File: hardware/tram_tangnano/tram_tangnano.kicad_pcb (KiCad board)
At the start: 4 copper layers, 93 x 26.7 mm, 61 parts, among them J1 Conn_01x01_SolderingPad, J10 Conn_01x01_SolderingPad, J11 Conn_01x01_SolderingPad, J12 Conn_01x01_SolderingPad, J13 Conn_01x01_SolderingPad, J14 Conn_01x01_SolderingPad, J15 Conn_01x01_SolderingPad, J16 Conn_01x01_SolderingPad, J17 Conn_01x01_SolderingPad, J18 Conn_01x01_SolderingPad, J19 Conn_01x01_SolderingPad, J2 Conn_01x01_SolderingPad, J20 Conn_01x01_SolderingPad, J21 Conn_01x01_SolderingPad, J22 Conn_01x01_SolderingPad, J23 Conn_01x01_SolderingPad, J24 Conn_01x01_SolderingPad, J3 Conn_01x04_Voltage, J4 Conn_01x01_SolderingPad, J5 Conn_01x01_SolderingPad, J6 Conn_01x01_SolderingPad, J7 Conn_01x01_SolderingPad, J8 Conn_01x01_SolderingPad, J9 Conn_01x01_SolderingPad, U1 Tang_Nano_20K, U10 TXU0202, U11 TXU0202, U12 TXU0202, U13 TXU0202, U20 TRAM, U4 SN74LVC2GU04, U6 SN74LVC1G06, U7 SN74LVC1G04

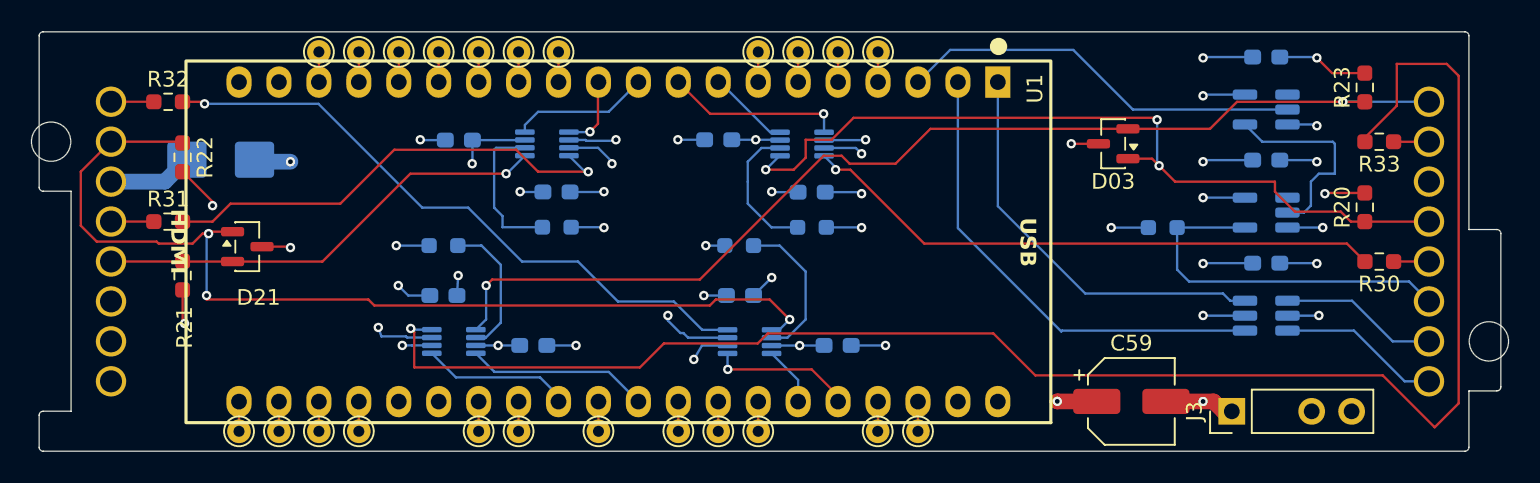
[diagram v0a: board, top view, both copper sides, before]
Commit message: temp
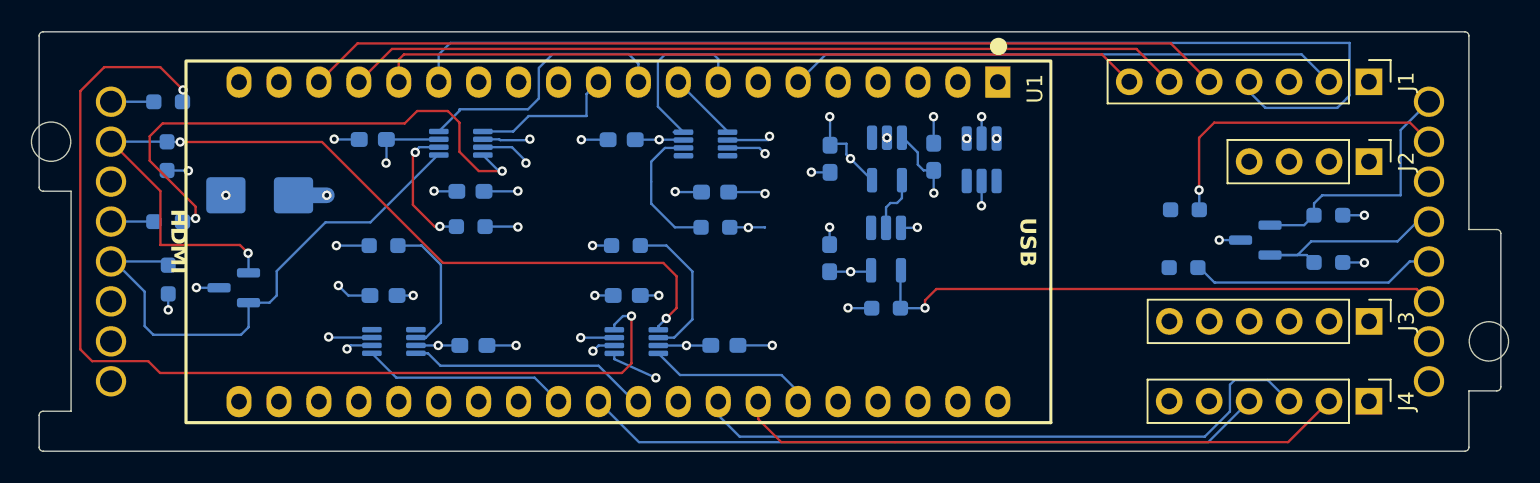
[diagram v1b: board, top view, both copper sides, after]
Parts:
- removed C59: 100µF, Capacitor_SMD:CP_Elec_5x3.9
- removed J10, J11, J12, J13, J14, J15, J16, J17, J18, J19, J20, J21, J22, J23, J24, J5, J6, J7, J8, J9: Conn_01x01_SolderingPad, Transputer:TestPoint_THTPad_D1.5mm_Drill0.7mm
- D03, D21, R20, R21, R22, R23, R30, R31, R32, R33: moved to B.Cu
- J1: value Conn_01x01_SolderingPad -> Conn_LED; footprint Transputer:TestPoint_THTPad_D1.5mm_Drill0.7mm -> Connector_PinHeader_2.54mm:PinHeader_1x07_P2.54mm_Vertical
- J2: value Conn_01x01_SolderingPad -> Conn_Event; footprint Transputer:TestPoint_THTPad_D1.5mm_Drill0.7mm -> Connector_PinHeader_2.54mm:PinHeader_1x04_P2.54mm_Vertical
- J3: value Conn_01x04_Voltage -> Conn_Link; footprint Transputer:PinHeader_1x04_P2.54mm_without_2 -> Connector_PinHeader_2.54mm:PinHeader_1x06_P2.54mm_Vertical
- J4: value Conn_01x01_SolderingPad -> Conn_Audio; footprint Transputer:TestPoint_THTPad_D1.5mm_Drill0.7mm -> Connector_PinHeader_2.54mm:PinHeader_1x06_P2.54mm_Vertical
- moved J4 38.9 mm to (214.6, 103.5), turned to -90 degrees
- moved J1 36.3 mm to (214.6, 83.2), turned to -90 degrees
- moved J2 35.6 mm to (214.6, 88.2), turned to -90 degrees
- moved C35 28.5 mm to (180.3, 88.1), turned to -90 degrees
- moved C34 28.5 mm to (180.3, 94.4), turned to 90 degrees
- moved U7 24.3 mm to (183.9, 88.1), turned to -90 degrees
- moved U6 24.3 mm to (183.9, 93.8), turned to -90 degrees
- moved C36 22.1 mm to (186.9, 87.9), turned to -90 degrees
- moved U4 20.6 mm to (190.0, 88.1), turned to 90 degrees
- moved R1 18.3 mm to (183.9, 97.6)
- moved R33 13.1 mm to (202.9, 91.3)
- moved R30 12.5 mm to (202.8, 95.0)
- moved D03 10.9 mm to (207.4, 93.2)
- moved J3 10.4 mm to (214.6, 98.4), turned to -90 degrees
- moved R23 8.45 mm to (212.0, 91.7), turned to 0 degrees
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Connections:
- net Net-(U1-25_IOB6A) renamed /ExtLink1In
- net Net-(U1-26_IOB6B) renamed /ExtLink1Out
- net Net-(U1-27_IOB8A) renamed /ExtLink0In
- net Net-(U1-28_IOB8B) renamed /ExtLink0Out
- net Net-(U1-41_IOB43A) renamed /ExtLink3In
- net Net-(U1-42_IOB42B) renamed /ExtLink3Out
- net Net-(U1-48_IOR49B) renamed /ExtLink4In
- net Net-(U1-49_IOR49A) renamed /ExtLink4Out
- J1 pad 1: Net-(J1-Pin_1) -> GND
- J2 pad 1: Net-(J2-Pin_1) -> GND
- J3 pad 3: +3.3V -> /ExtLink2Out
- J3 pad 4: +5V -> GND
- J4 pad 1: Net-(J4-Pin_1) -> unconnected-(J4-Pin_1-Pad1)
- R20 pad 1: Net-(D03-A1) -> Net-(D03-A2)
- R23 pad 1: Net-(D03-A2) -> Net-(D03-A1)
- U1 pad 12: Net-(J18-Pin_1) -> /ExtLink2In
- U1 pad 13: Net-(J19-Pin_1) -> /ExtLink2Out
- U1 pad 14: Net-(J20-Pin_1) -> /EventReq
- U1 pad 15: Net-(J21-Pin_1) -> /LED2
- U1 pad 16: Net-(J22-Pin_1) -> /LED5
- U1 pad 17: Net-(J23-Pin_1) -> /LED4
- U1 pad 18: Net-(J24-Pin_1) -> /LED3
- U1 pad 21: Net-(J13-Pin_1) -> unconnected-(U1-52_IOR39A-Pad21)
- U1 pad 22: Net-(J12-Pin_1) -> unconnected-(U1-53_IOR38B-Pad22)
- U1 pad 23: Net-(J11-Pin_1) -> /ExtLink5Out
- U1 pad 24: Net-(J10-Pin_1) -> /ExtLink5In
- U1 pad 27: Net-(J9-Pin_1) -> unconnected-(U1-79_IOT27B-Pad27)
- U1 pad 28: Net-(J8-Pin_1) -> /EventAck
- U1 pad 30: Net-(J7-Pin_1) -> /AUDIO_I2S_LRCK
- U1 pad 32: Net-(J6-Pin_1) -> /AUDIO_PA_EN
- U1 pad 33: Net-(J5-Pin_1) -> /AUDIO_I2S_DIN
- U1 pad 34: Net-(J4-Pin_1) -> /AUDIO_I2S_BCLK
- U1 pad 37: Net-(J2-Pin_1) -> unconnected-(U1-80_IOT27A-Pad37)
- U1 pad 38: Net-(J1-Pin_1) -> /EventWaiting
- U1 pad 4: Net-(J14-Pin_1) -> unconnected-(U1-85_IOT4B-Pad4)
- U1 pad 5: Net-(J15-Pin_1) -> unconnected-(U1-77_IOT30A-Pad5)
- U1 pad 6: Net-(J16-Pin_1) -> /LED0
- U1 pad 7: Net-(J17-Pin_1) -> /LED1
- U10 pad 5: Net-(D03-A1) -> Net-(D03-A2)
- U13 pad 5: Net-(D03-A2) -> Net-(D03-A1)
- U20 pad 13: Net-(D03-A1) -> Net-(D03-A2)
- U20 pad 16: Net-(D03-A2) -> Net-(D03-A1)
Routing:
- net +3.3V: track 32.8 -> 161.6 mm, vias 10 -> 9
- net Net-(U13-A2Y): track 105.5 -> 0.00 mm, vias 1 -> 0
- net +5V: track 60.2 -> 161.2 mm, vias 17 -> 16
- net /EventAck: track 0.00 -> 91.1 mm
- net /LED2: track 0.00 -> 71.1 mm
- net /ExtLink5In: track 0.00 -> 65.1 mm
- net /EventReq: track 0.00 -> 63.5 mm
- net /EventWaiting: track 0.00 -> 61.9 mm
- net /ExtLink5Out: track 0.00 -> 61.6 mm
- net /LED3: track 0.00 -> 58.6 mm
- net Net-(D03-A2): track 69.7 -> 14.0 mm, vias 2 -> 0
- net /LED4: track 0.00 -> 53.3 mm
- net /LED5: track 0.00 -> 48.7 mm
- net /AUDIO_I2S_LRCK: track 0.00 -> 43.5 mm
- net /AUDIO_I2S_DIN: track 0.00 -> 40.8 mm
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- removed copper zone on In2.Cu, net +3.3V
- removed copper zone on In2.Cu, net +5V
